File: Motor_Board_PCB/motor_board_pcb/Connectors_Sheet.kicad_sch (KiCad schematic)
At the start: 10 parts, among them J11 CSP-USC16-TR, J6 Screw_Terminal_01x04, J7 Conn_01x03, J8 Conn_01x02

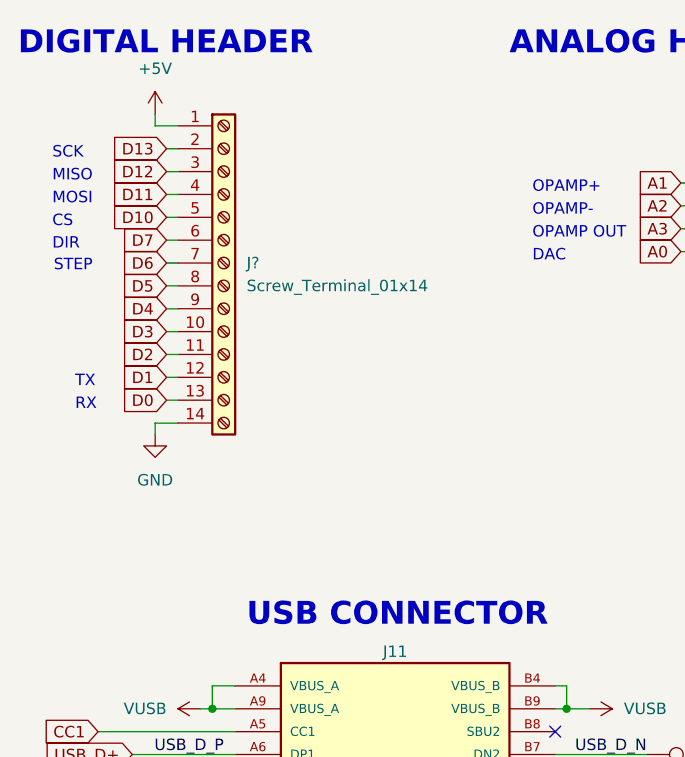
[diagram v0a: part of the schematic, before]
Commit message: Motor Board Initial Layout
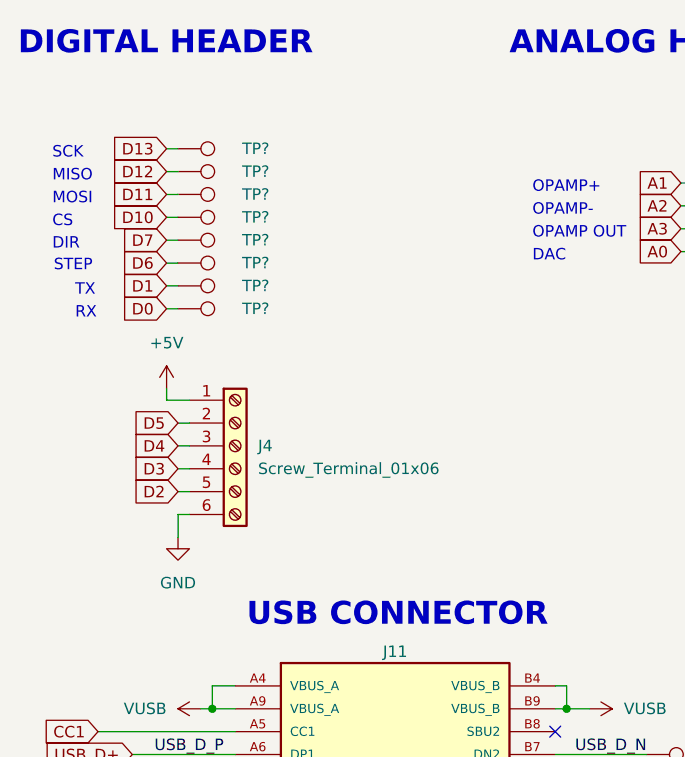
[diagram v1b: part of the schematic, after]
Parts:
- removed J?: Screw_Terminal_01x14, Connector_PinHeader_2.54mm:PinHeader_1x14_P2.54mm_Vertical, symbol Connector:Screw_Terminal_01x14
- added J4: Screw_Terminal_01x06, Connector_PinHeader_2.54mm:PinHeader_1x06_P2.54mm_Vertical, symbol Connector:Screw_Terminal_01x06
- added TP? (x8): TestPoint, TestPoint:TestPoint_Pad_D1.0mm, symbol Connector:TestPoint
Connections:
- net +5V: now also J4.1 (Pin_1)
- net D0: now also TP?.1
- net D1: now also TP?.1
- net D10: now also TP?.1
- net D11: now also TP?.1
- net D12: now also TP?.1
- net D13: now also TP?.1
- net D2: now also J4.5 (Pin_5)
- net D3: now also J4.4 (Pin_4)
- net D4: now also J4.3 (Pin_3)
- net D5: now also J4.2 (Pin_2)
- net D6: now also TP?.1
- net D7: now also TP?.1
- net GND: now also J4.6 (Pin_6)
